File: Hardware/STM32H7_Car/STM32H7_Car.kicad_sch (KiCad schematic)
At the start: 37 parts, among them J1 L_MOTOR, J2 R_MOTOR, J3 L_ENC, J4 R_ENC, J5 L_ADC, J6 IR_ADC, J7 IMU, J8 OLED, J9 WIFI, U1 TPS54627DDAR, U2 TPS54325PWPR

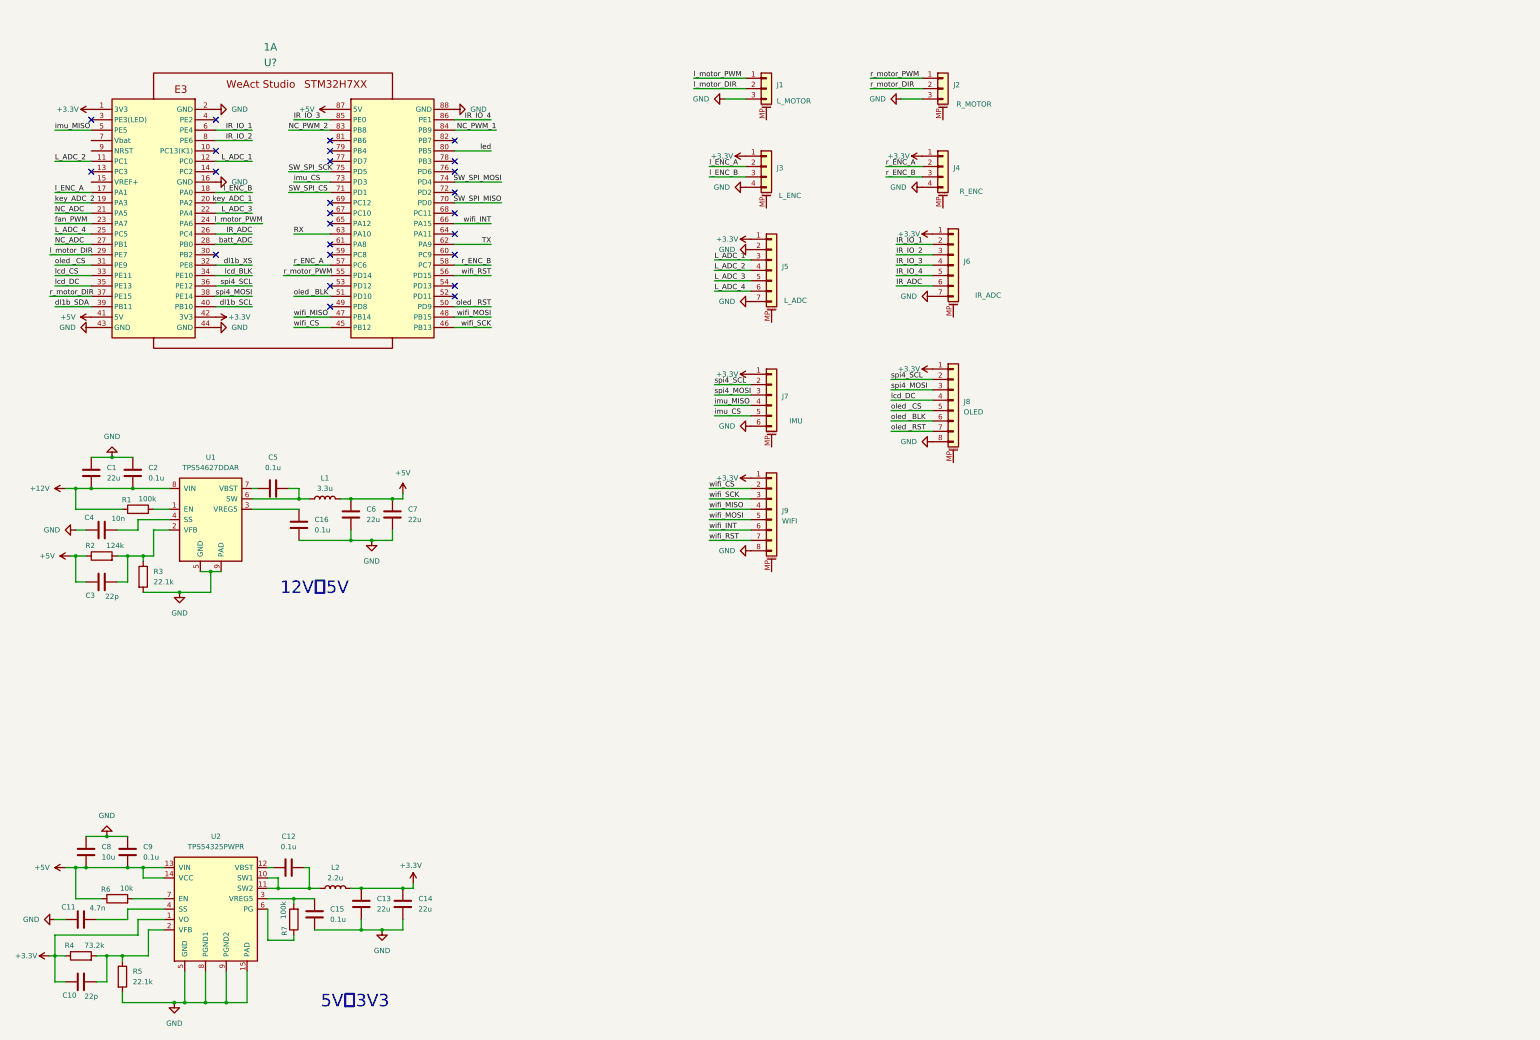
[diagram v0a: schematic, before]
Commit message: 归档硬件设计与项目参考资料快照
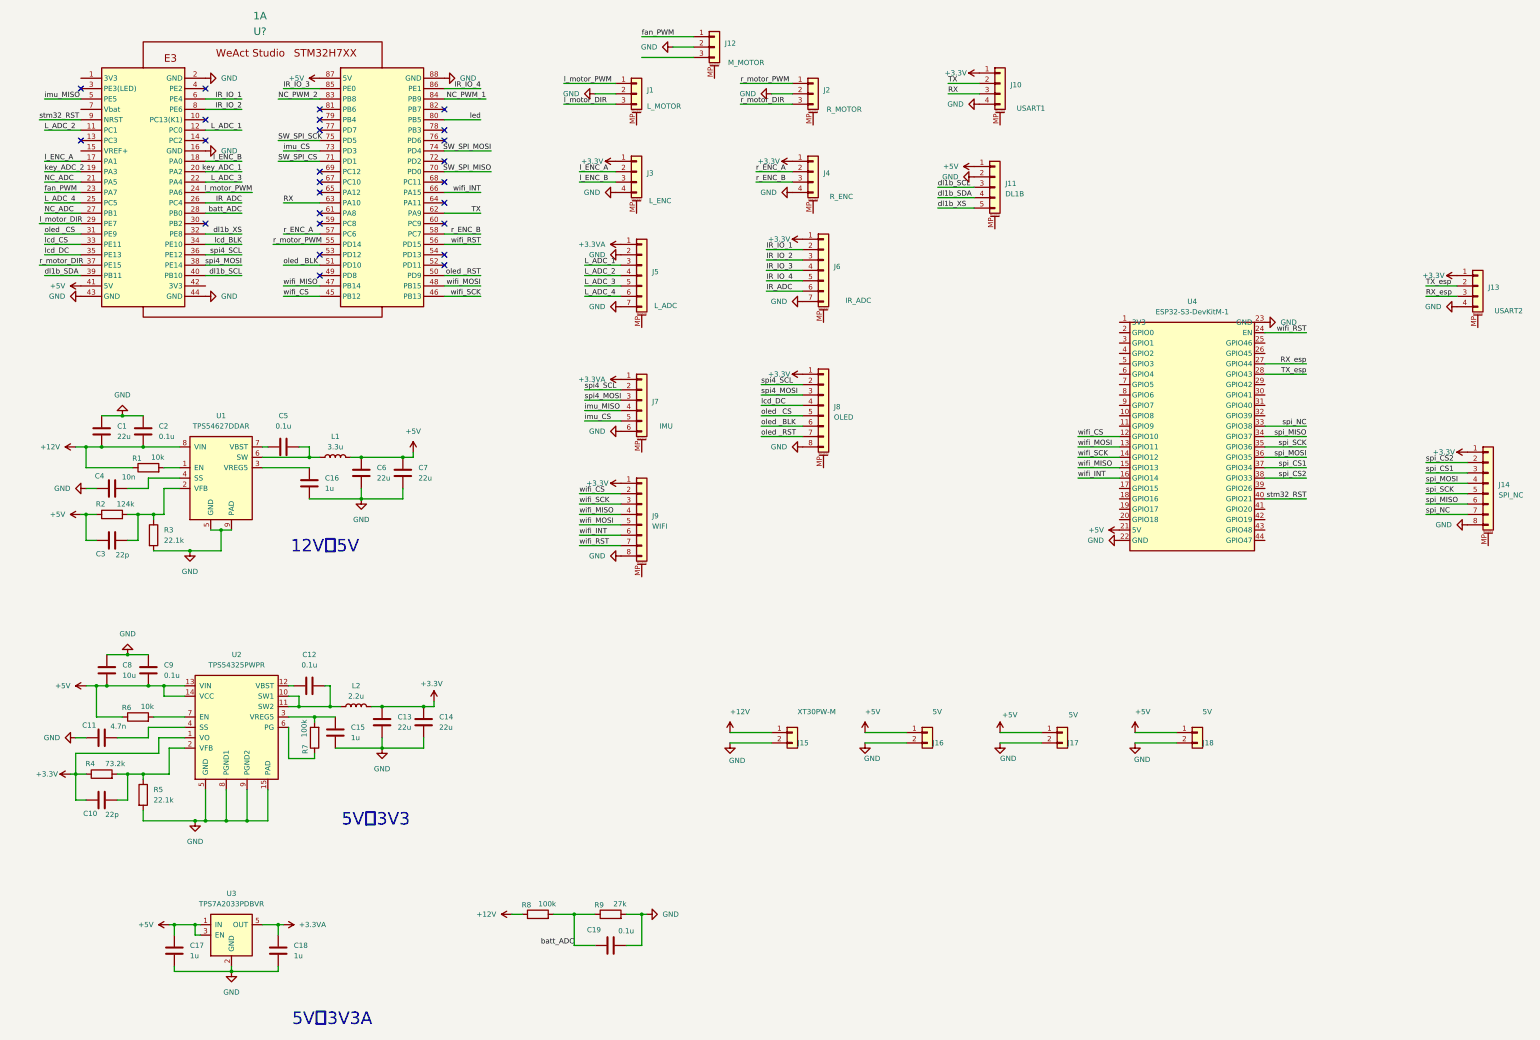
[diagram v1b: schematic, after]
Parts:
- added C17, C18: 1u, Capacitor_SMD:C_0603_1608Metric, symbol Device:C
- added C19: 0.1u, Capacitor_SMD:C_0603_1608Metric, symbol Device:C
- added J10: USART1, Connector_PinHeader_2.54mm:PinHeader_1x04_P2.54mm_Vertical, symbol Connector_Generic_MountingPin:Conn_01x04_MountingPin
- added J11: DL1B, Connector_PinHeader_2.54mm:PinHeader_1x05_P2.54mm_Vertical, symbol Connector_Generic_MountingPin:Conn_01x05_MountingPin
- added J12: M_MOTOR, Connector_PinHeader_2.54mm:PinHeader_1x03_P2.54mm_Vertical, symbol Connector_Generic_MountingPin:Conn_01x03_MountingPin
- added J13: USART2, Connector_PinHeader_2.54mm:PinHeader_1x04_P2.54mm_Vertical, symbol Connector_Generic_MountingPin:Conn_01x04_MountingPin
- added J14: SPI_NC, Connector_PinHeader_2.54mm:PinHeader_1x08_P2.54mm_Vertical, symbol Connector_Generic_MountingPin:Conn_01x08_MountingPin
- added J15: XT30PW-M, Connector_AMASS:AMASS_XT30PW-M_1x02_P2.50mm_Horizontal, symbol Connector_Generic:Conn_01x02
- added J16, J17, J18: 5V, Connector_PinHeader_2.54mm:PinHeader_1x02_P2.54mm_Vertical, symbol Connector_Generic:Conn_01x02
- added R8: 100k, Resistor_SMD:R_0603_1608Metric, symbol Device:R
- added R9: 27k, Resistor_SMD:R_0603_1608Metric, symbol Device:R
- added U3: TPS7A2033PDBVR, Library:SOT-23-5, symbol Library:TPS7A2033PDBVR
- added U4: ESP32-S3-DevKitM-1, Library:ESP32-S3-DevKitM-1, symbol Library:ESP32-S3-DevKitM-1
- C1, C13, C14, C6, C7, C8: footprint Library:TI_DDA0008A_SO-PowerPAD-8 -> Capacitor_SMD:C_0805_2012Metric
- C10, C11, C12, C2, C3, C4, C5, C9: footprint (none) -> Capacitor_SMD:C_0603_1608Metric
- C15, C16: value 0.1u -> 1u; footprint (none) -> Capacitor_SMD:C_0603_1608Metric
- J1, J2: footprint Connector_Audio:Jack_XLR_Neutrik_NC3FBV1-0_Vertical -> Connector_PinHeader_2.54mm:PinHeader_1x03_P2.54mm_Vertical
- J3, J4: footprint (none) -> Connector_PinHeader_1.27mm:PinHeader_1x04_P1.27mm_Vertical
- J5, J6: footprint (none) -> Connector_PinHeader_2.54mm:PinHeader_1x07_P2.54mm_Vertical
- J7: footprint (none) -> Connector_PinHeader_2.54mm:PinHeader_1x06_P2.54mm_Vertical
- J8: footprint (none) -> Connector_PinHeader_2.54mm:PinHeader_1x08_P2.54mm_Vertical
- J9: footprint (none) -> Connector_PinHeader_2.54mm:PinHeader_2x04_P2.54mm_Vertical
- L1: footprint (none) -> Library:L_Molded_5x5mm_FEXL0530A_ZD0520; LCSC (none) -> C5378512
- L2: footprint (none) -> Library:L_Molded_5x5mm_FEXL0530A_ZD0520; LCSC (none) -> C46956540
- R1: value 100k -> 10k; footprint (none) -> Resistor_SMD:R_0603_1608Metric
- R2, R3, R4, R5, R6, R7: footprint (none) -> Resistor_SMD:R_0603_1608Metric
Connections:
- net +12V: now also J15.1 (Pin_1), R8.1
- net +3.3V: now also J10.1 (Pin_1), J13.1 (Pin_1), J14.1 (Pin_1); no longer 1.1 (3V3), 1.42 (3V3), J5.1 (Pin_1), J7.1 (Pin_1)
- net +5V: now also C17.1, J11.1 (Pin_1), J16.1 (Pin_1), J17.1 (Pin_1), J18.1 (Pin_1), U3.1 (IN), U3.3 (EN), U4.21 (5V)
- net GND: now also J1.2 (Pin_2), J2.2 (Pin_2), C17.2, C18.2, C19.1, J10.4 (Pin_4), J11.2 (Pin_2), J12.2 (Pin_2), J13.4 (Pin_4), J14.8 (Pin_8), J15.2 (Pin_2), J16.2 (Pin_2), J17.2 (Pin_2), J18.2 (Pin_2), R9.2, U3.2 (GND), U4.22 (GND), U4.23 (GND); no longer J1.3 (Pin_3), J2.3 (Pin_3)
- net RX: now also J10.3 (Pin_3)
- net TX: now also J10.2 (Pin_2)
- net batt_ADC: now also C19.2, R8.2, R9.1
- net dl1b_SCL: now also J11.3 (Pin_3)
- net dl1b_SDA: now also J11.4 (Pin_4)
- net dl1b_XS: now also J11.5 (Pin_5)
- net fan_PWM: now also J12.1 (Pin_1)
- net l_motor_DIR: now also J1.3 (Pin_3); no longer J1.2 (Pin_2)
- net r_motor_DIR: now also J2.3 (Pin_3); no longer J2.2 (Pin_2)
- net wifi_CS: now also U4.12 (GPIO10)
- net wifi_INT: now also U4.16 (GPIO14)
- net wifi_MISO: now also U4.15 (GPIO13)
- net wifi_MOSI: now also U4.13 (GPIO11)
- net wifi_RST: now also U4.24 (EN)
- net wifi_SCK: now also U4.14 (GPIO12)
- net stm32_RST: now reaches 1.9 (NRST)
- net stm32_RST: now also U4.40 (GPIO21)
- new net +3.3VA: C18.1, J5.1 (Pin_1), J7.1 (Pin_1), U3.5 (OUT)
- new net RX_esp: J13.3 (Pin_3), U4.27 (GPIO44)
- new net TX_esp: J13.2 (Pin_2), U4.28 (GPIO43)
- new net spi_CS1: J14.3 (Pin_3), U4.37 (GPIO34)
- new net spi_CS2: J14.2 (Pin_2), U4.38 (GPIO33)
- new net spi_MISO: J14.6 (Pin_6), U4.34 (GPIO37)
- new net spi_MOSI: J14.4 (Pin_4), U4.36 (GPIO35)
- new net spi_NC: J14.7 (Pin_7), U4.33 (GPIO38)
- new net spi_SCK: J14.5 (Pin_5), U4.35 (GPIO36)
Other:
- note added: "5V转3V3A"
- moved on the sheet: 1A, C1, C10, C11, C12, C13, C14, C15, C16, C2, C3, C4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
